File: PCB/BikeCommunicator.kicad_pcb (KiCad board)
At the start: 2 copper layers, 60 x 60 mm, 27 parts, among them J1 Barrel_Jack_Switch, J2 USB_B_Micro, J3 Conn_01x04, J4 Conn_01x02, SW1 SW_SPST_LED, SW2 SW_SPST_LED, SW3 SW_SPST_LED, SW4 SW_SPST_LED, SW5 SW_DPDT_x2, U1 HW-108_DC-DC, U2 HTCC-AB01

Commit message: Updated PCB project file
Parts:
- R1: value R -> 0R
- R2: value R -> 220R
- R3, R4, R7, R8: value R -> 4k7
- R5, R6: value R -> 120R
- SW1: value SW_SPST_LED -> SW_SPST_LED_Green
- SW2: value SW_SPST_LED -> SW_SPST_LED_Blue
- SW3: value SW_SPST_LED -> SW_SPST_LED_Yellow
- SW4: value SW_SPST_LED -> SW_SPST_LED_Red

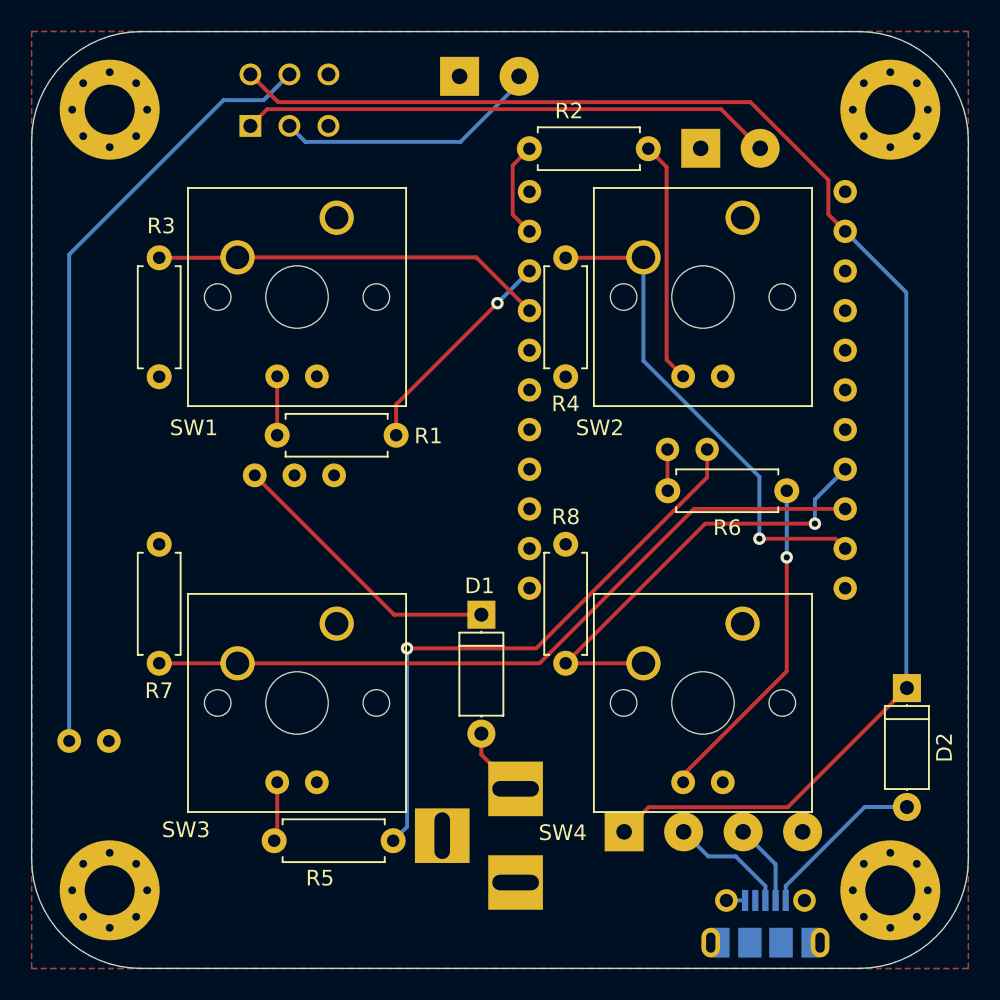
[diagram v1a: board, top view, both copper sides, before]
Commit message: Major PCB fix
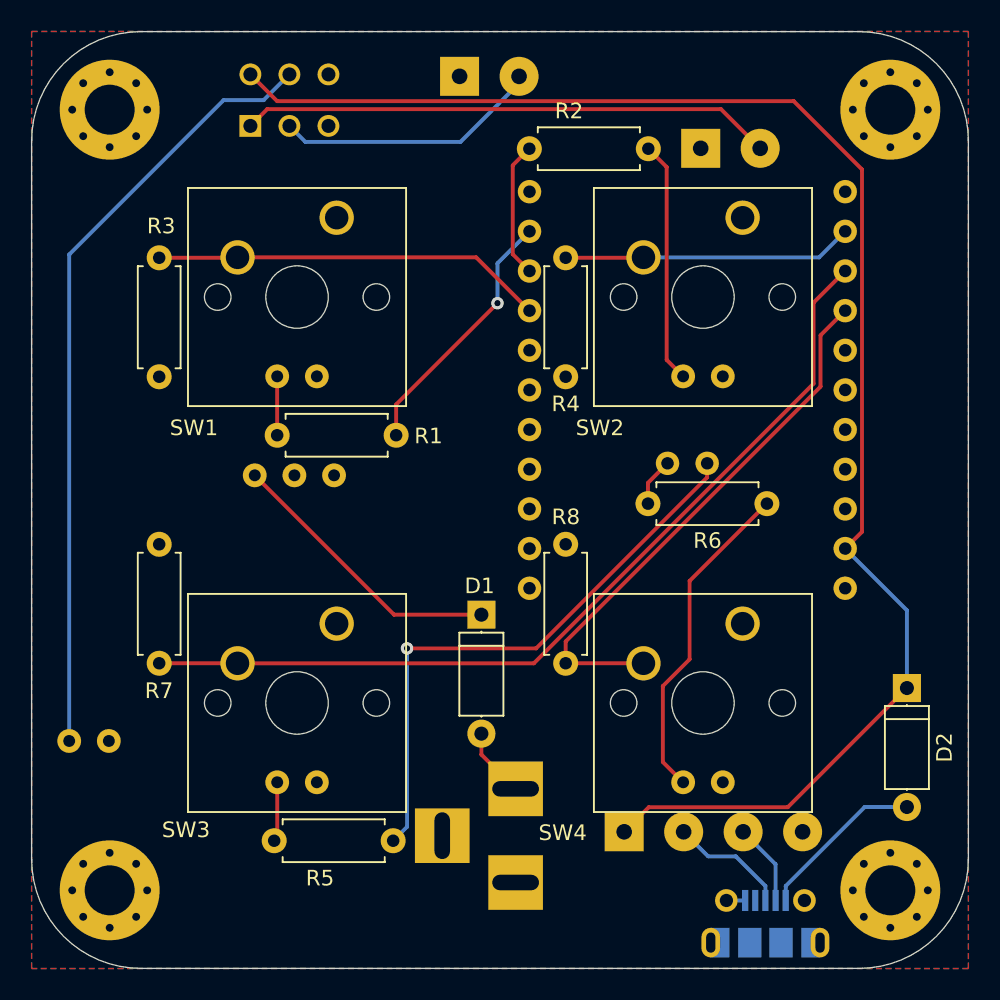
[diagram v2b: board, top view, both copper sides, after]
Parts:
- moved R6 1.51 mm to (137.1, 90.2)
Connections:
- U2 pad 10: /LED2 -> /LED1
- U2 pad 12: -BATT -> Net-(U2-Pad12)
- U2 pad 13: +5V -> /BTN2
- U2 pad 14: Net-(U2-Pad14) -> /BTN3
- U2 pad 15: Net-(U2-Pad15) -> /BTN4
- U2 pad 19: /BTN4 -> Net-(U2-Pad19)
- U2 pad 20: /BTN3 -> Net-(U2-Pad20)
- U2 pad 21: /BTN2 -> +5V
- U2 pad 22: Net-(U2-Pad22) -> -BATT
- U2 pad 9: /LED1 -> /LED2
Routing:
- net /BTN2: track 31.8 -> 18.2 mm, vias 1 -> 0
- net /BTN3: track 48.0 -> 57.4 mm
- net /BTN4: track 28.9 -> 35.0 mm, vias 1 -> 0
- net +5V: track 96.4 -> 98.9 mm
- net /LED1: track 14.1 -> 16.6 mm
- net /LED2: track 6.18 -> 8.72 mm
- net /LED3: track 38.2 -> 37.3 mm
- net Net-(R6-Pad1): track 21.4 -> 21.1 mm, vias 1 -> 0
